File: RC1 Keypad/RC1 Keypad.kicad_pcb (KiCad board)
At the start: 2 copper layers, 73 x 122.6 mm, 26 parts, among them J1 KB, SW1 Ø, SW10 3, SW11 A, SW12 DA, SW13 4, SW14 B, SW15 +, SW16 5, SW17 C, SW18 GO, SW19 6, SW2 7, SW20 D, SW21 PC, SW22 SST, SW23 RS, SW24 ST, SW3 E, SW4 1, SW5 8, SW6 F, SW7 2, SW8 9, SW9 AD

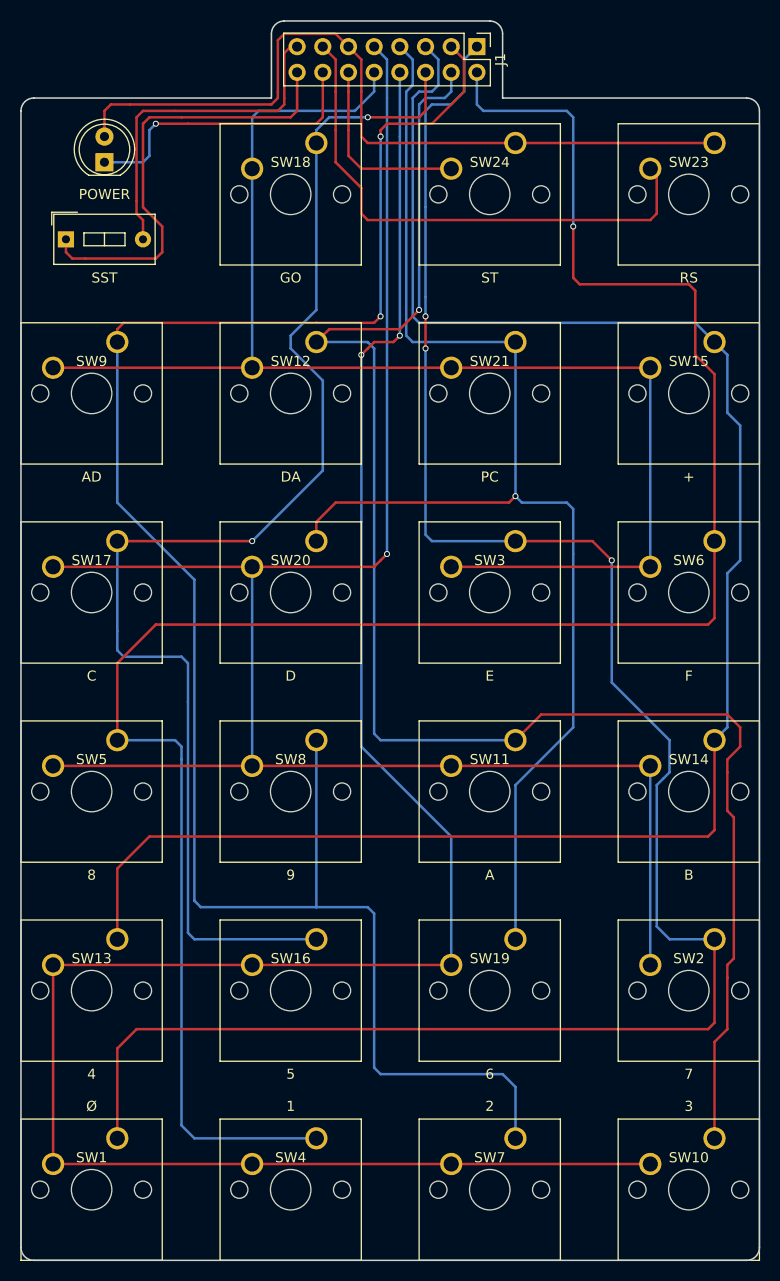
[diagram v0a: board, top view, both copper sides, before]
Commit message: Keypad SX layout done
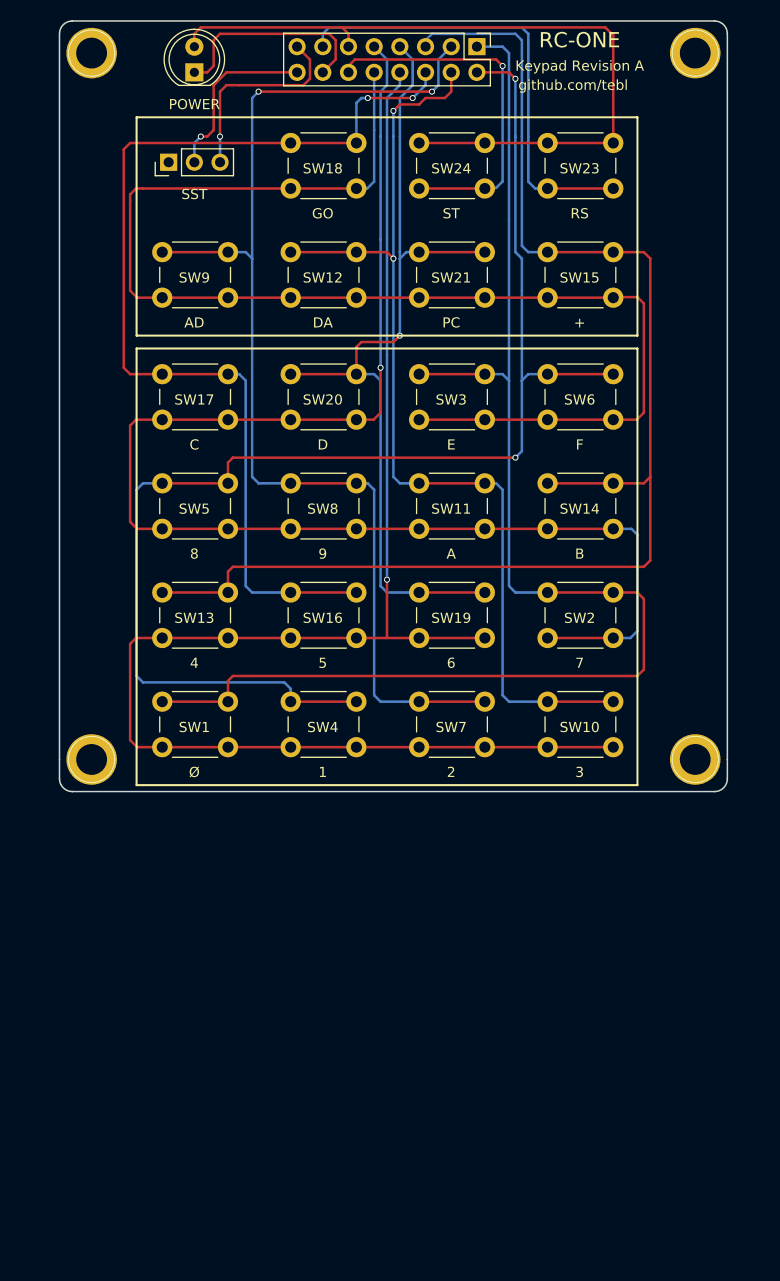
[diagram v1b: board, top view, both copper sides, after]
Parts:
- added M1: Mounting, Mounting:1pin, F.Cu at (91.4, 58.4)
- added M2: Mounting, Mounting:1pin, F.Cu at (151.1, 58.4)
- added M3: Mounting, Mounting:1pin, F.Cu at (91.4, 128.3)
- added M4: Mounting, Mounting:1pin, F.Cu at (151.1, 128.3)
- SW1, SW10, SW11, SW12, SW13, SW14, SW15, SW16, SW17, SW18, SW19, SW2, SW20, SW21, SW23, SW24, SW3, SW4, SW5, SW6, SW7, SW8, SW9: footprint Button_Switch_Keyboard:SW_Cherry_MX_1.00u_PCB -> Buttons_Switches_THT:SW_PUSH_6mm
- SW22: footprint Buttons_Switches_THT:SW_DIP_x1_W7.62mm_Slide -> Pin_Headers:Pin_Header_Straight_1x03_Pitch2.54mm
- moved SW10 46.2 mm to (136.5, 122.6)
- moved SW7 44.2 mm to (123.8, 122.6)
- moved SW1 43.4 mm to (98.4, 122.6)
- moved SW4 43.3 mm to (111.1, 122.6)
- moved SW2 38.1 mm to (136.5, 111.8)
- moved SW19 35.6 mm to (123.8, 111.8)
- moved SW13 34.6 mm to (98.4, 111.8)
- moved SW16 34.4 mm to (111.1, 111.8)
- moved SW14 30.3 mm to (136.5, 101.0)
- moved SW11 27.1 mm to (123.8, 101.0)
- moved SW5 25.8 mm to (98.4, 101.0)
- moved SW8 25.5 mm to (111.1, 101.0)
- moved SW6 23.3 mm to (136.5, 90.2)
- moved SW3 19.1 mm to (123.8, 90.2)
- moved SW15 18.8 mm to (136.5, 78.1)
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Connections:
- net /2A0 renamed /PA0
- net /2A1 renamed /PA1
- net /2A2 renamed /PA2
- net /2A3 renamed /PA3
- net /2A4 renamed /PA4
- net /2A5 renamed /PA5
- net /2A6 renamed /PA6
- net /ROW_0 renamed /ROW2
- net /ROW_1 renamed /ROW1
- net /ROW_2 renamed /ROW0
- SW22 pad 1: /SST_IN -> (no net)
- SW22 pad 2: /SST_OUT -> /SST_IN
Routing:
- net /PA4: track 189.3 -> 114.0 mm
- net /PA5: track 201.3 -> 133.3 mm, vias 1 -> 2
- net /PA3: track 161.7 -> 97.9 mm, vias 1 -> 2
- net /ROW0: track 212.8 -> 149.4 mm, vias 2 -> 1
- net /PA6: track 193.5 -> 136.4 mm, vias 3 -> 0
- net /PA0: track 129.5 -> 85.8 mm
- net /PA2: track 177.9 -> 135.3 mm
- net /ROW1: track 182.7 -> 141.2 mm
- net /PA1: track 132.6 -> 101.8 mm
- net /SST_IN: track 44.4 -> 17.6 mm, vias 0 -> 1
- net /ST: track 18.9 -> 36.4 mm, vias 0 -> 1
- net /SST_OUT: track 34.1 -> 20.1 mm, vias 0 -> 1
- net /ROW2: track 138.2 -> 129.7 mm
- net /LED: track 29.5 -> 21.0 mm, vias 1 -> 0
- net /RS: track 52.5 -> 45.4 mm
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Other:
- board size 73 x 122.6 mm -> 66 x 76.2 mm
- board text added: "Keypad Revision A"
- board text added: "RC-ONE"
- board text added: "github.com/tebl"
